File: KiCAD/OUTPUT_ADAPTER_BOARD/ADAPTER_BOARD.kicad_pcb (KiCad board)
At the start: 2 copper layers, 58 x 107 mm, 81 parts, among them Q1 Q_NPN_CBE, Q10 Q_NPN_CBE, Q11 Q_NPN_CBE, Q12 Q_NPN_CBE, Q13 Q_NPN_CBE, Q14 Q_NPN_CBE, Q15 Q_NPN_CBE, Q16 Q_NPN_CBE, Q17 Q_NPN_CBE, Q18 Q_NPN_CBE, Q19 Q_NPN_CBE, Q2 Q_NPN_CBE, Q20 Q_NPN_CBE, Q21 Q_NPN_CBE, Q22 Q_NPN_CBE, Q23 Q_NPN_CBE, Q24 Q_NPN_CBE, Q3 Q_NPN_CBE, Q4 Q_NPN_CBE, Q5 Q_NPN_CBE, Q6 Q_NPN_CBE, Q7 Q_NPN_CBE, Q8 Q_NPN_CBE, Q9 Q_NPN_CBE

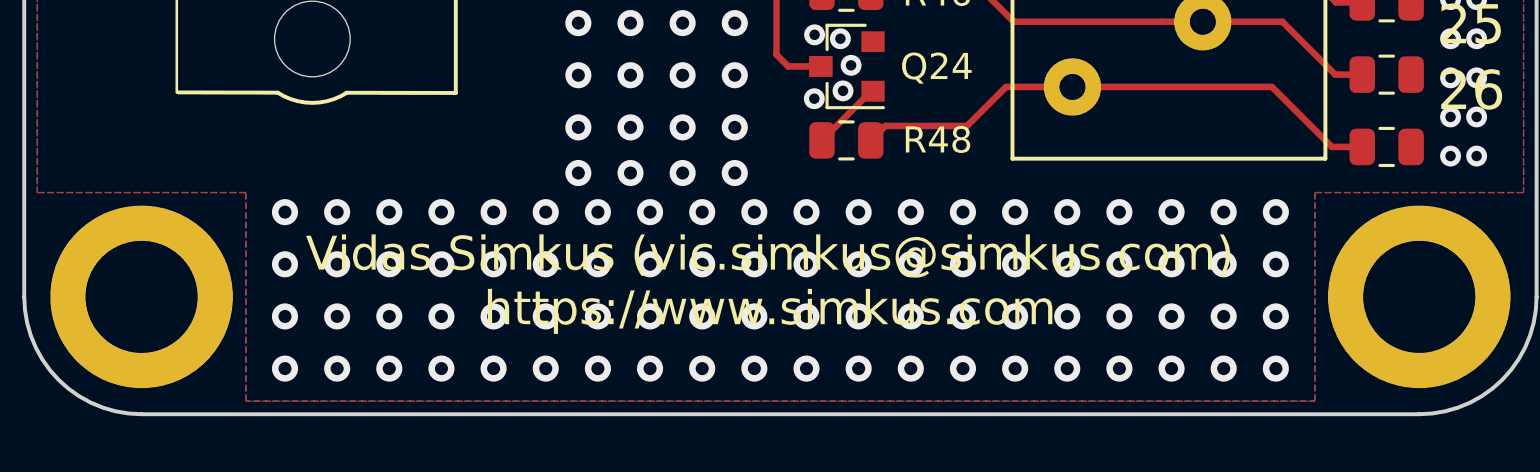
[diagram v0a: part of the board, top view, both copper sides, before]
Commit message: Text label updates.
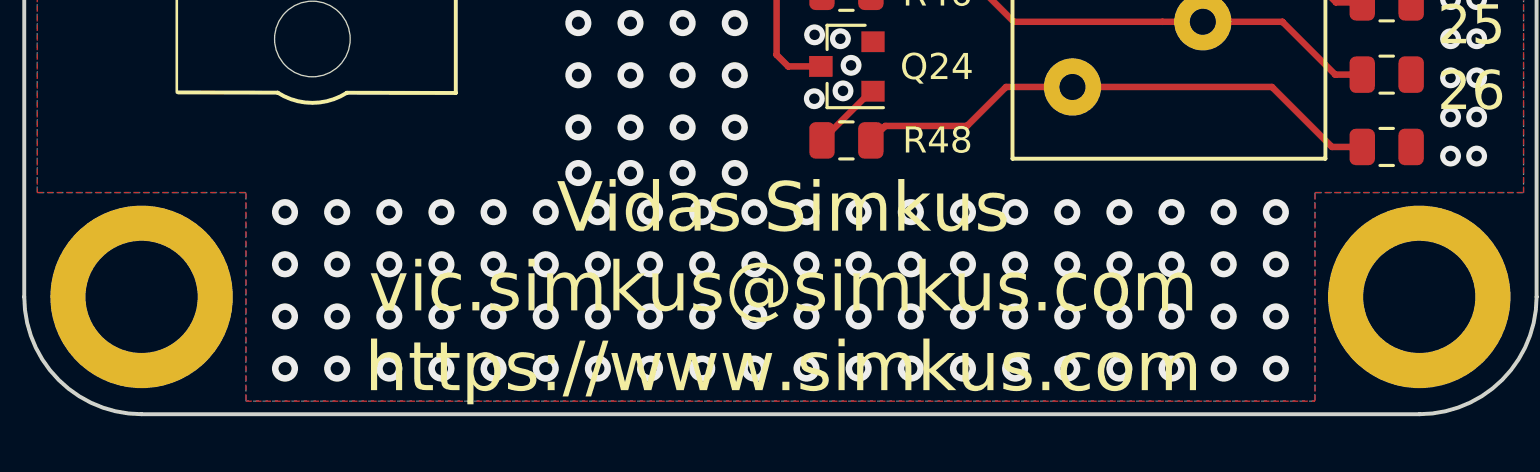
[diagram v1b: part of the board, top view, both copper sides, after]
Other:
- board text added: "Vidas Simkus vic.simkus@simkus.com https://www.simkus.com"
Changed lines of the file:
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@@
   )
   (gr_text "Vidas Simkus (vic.simkus@simkus.com)\nhttps://www.simkus.com" (at 55.8 75.2 270) (layer B.SilkS)
-    (effects (font (size 1.3 1.3) (thickness 0.2)) (justify mirror))
+    (effects (font (size 2 2) (thickness 0.3)) (justify mirror))
   )
-  (gr_text "Vidas Simkus (vic.simkus@simkus.com)\nhttps://www.simkus.com" (at 79.1 124.4) (layer F.SilkS)
-    (effects (font (size 1.3 1.3) (thickness 0.2)))
+  (gr_text "Vidas Simkus\nvic.simkus@simkus.com\nhttps://www.simkus.com" (at 79.61 124.64) (layer F.SilkS)
+    (effects (font (size 1.9 1.9) (thickness 0.35)))
   )
   (gr_text 12 (at 106 75.059991) (layer F.SilkS)
